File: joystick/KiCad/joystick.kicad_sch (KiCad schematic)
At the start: 5 parts, among them J2 Conn_01x05_Pin, U1 COM-09032

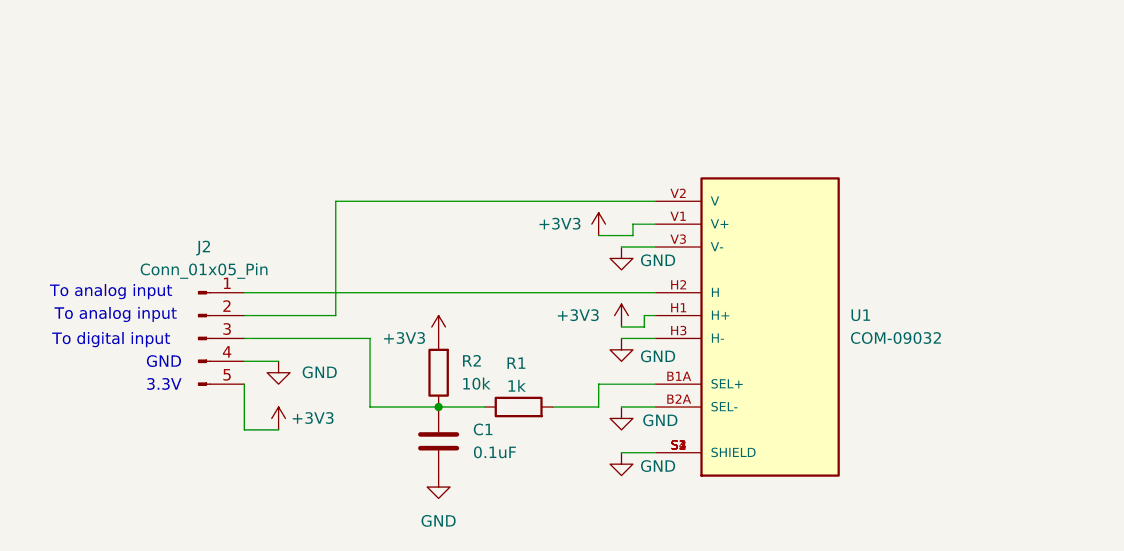
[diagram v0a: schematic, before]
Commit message: Deployed 1b09535 with MkDocs version: 1.6.0
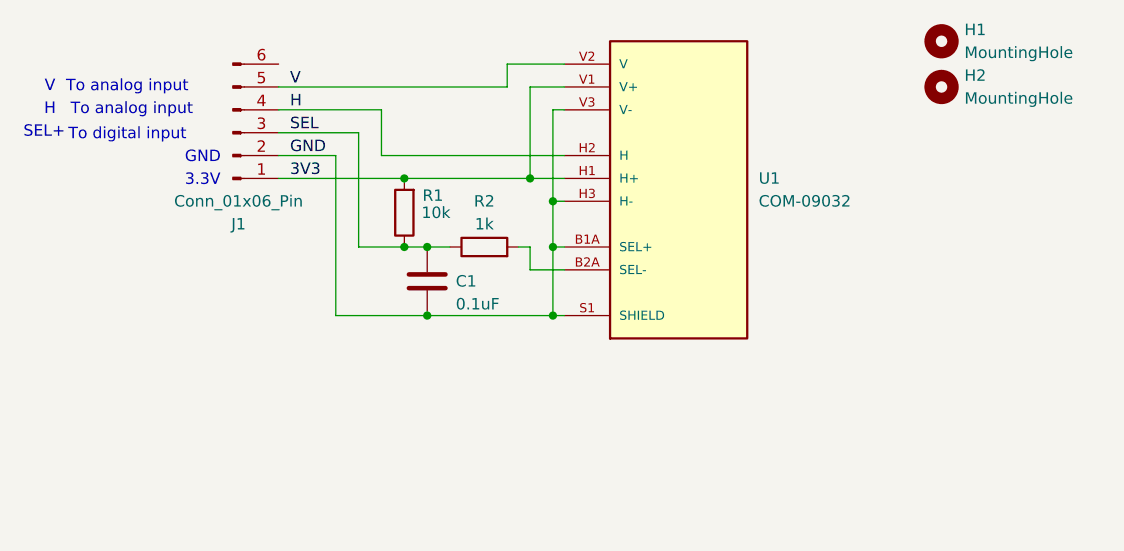
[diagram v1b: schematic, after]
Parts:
- removed J2: Conn_01x05_Pin, Connector_PinHeader_2.54mm:PinHeader_1x05_P2.54mm_Vertical, symbol Connector:Conn_01x05_Pin
- added H1, H2: MountingHole, MountingHole:MountingHole_3.2mm_M3_DIN965, symbol Mechanical:MountingHole
- added J1: Conn_01x06_Pin, Connector_PinHeader_2.54mm:PinHeader_1x06_P2.54mm_Vertical, symbol Connector:Conn_01x06_Pin
- U1: footprint XDCR_COM-09032 -> COM-09032:XDCR_COM-09032; Availability (none) -> In Stock; Check_prices (none) -> https://www.snapeda.com/parts/COM-09032/SparkFun/view-part/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; Description_1 (none) -> Joystick, 2 - Axis Analog (Resistive) Output; MF (none) -> SparkFun Electronics; MP (none) -> COM-09032; Package (none) -> Package; Price (none) -> None; SnapEDA_Link (none) -> https://www.snapeda.com/parts/COM-09032/SparkFun/view-part/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
- renumbered R2 to R1, R1 to R2
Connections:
- net GND: now also U1.B1A (SEL+), J1.2 (Pin_2); no longer U1.B2A (SEL-)
- net SEL: now reaches C1.1, R1.1, R2.1
- net SEL: now also J1.3 (Pin_3)
- net at R2.2: now also U1.B2A (SEL-); no longer U1.B1A (SEL+)
- net H: now reaches U1.H2 (H)
- net H: now also J1.4 (Pin_4)
- net V: now reaches U1.V2 (V)
- net V: now also J1.5 (Pin_5)
- net +3V3 renamed 3V3
- net 3V3: now also J1.1 (Pin_1)
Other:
- note added: "H"
- note added: "SEL+"
- note added: "V"
- moved on the sheet: C1, R1, R2
